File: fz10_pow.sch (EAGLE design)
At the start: 83 parts

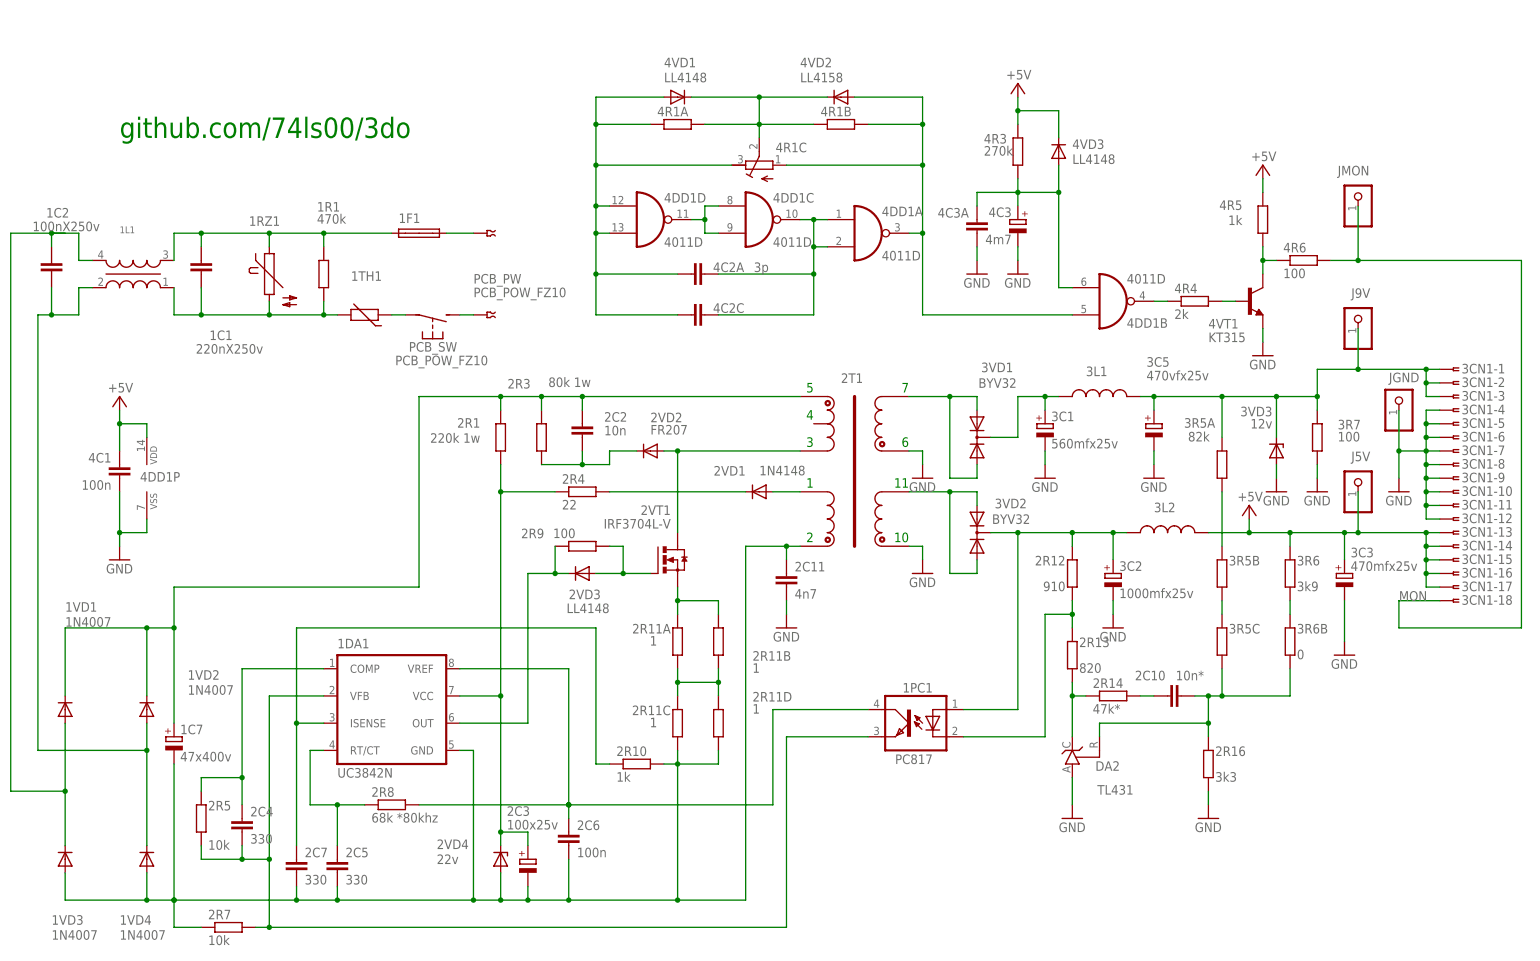
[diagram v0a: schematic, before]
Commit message: .
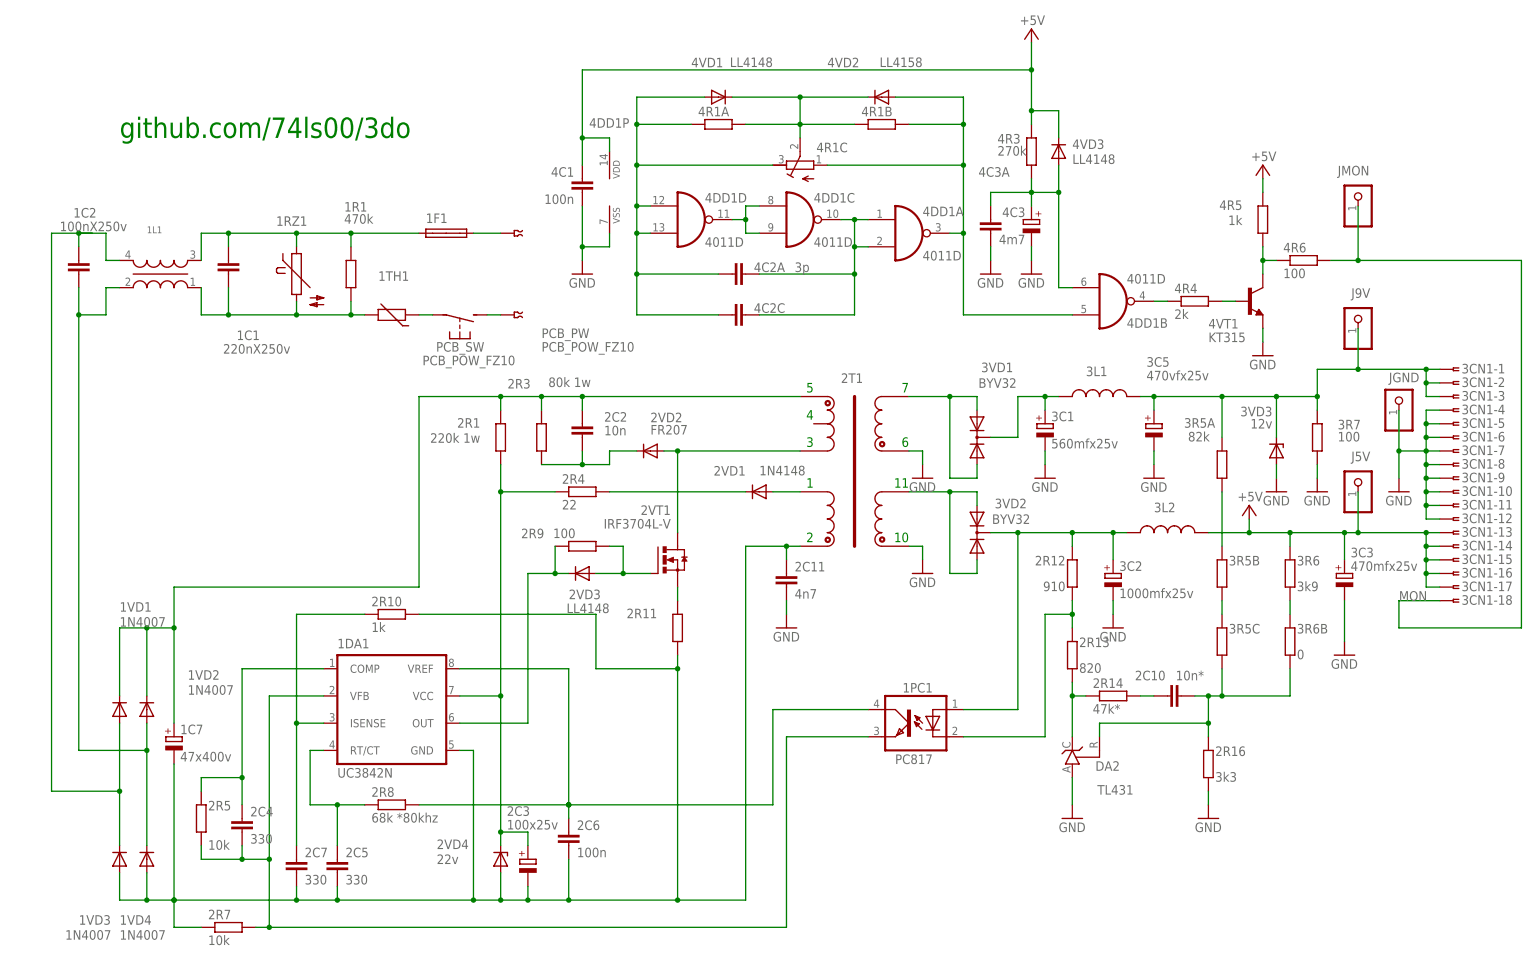
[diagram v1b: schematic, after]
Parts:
- removed 2R11A, 2R11B, 2R11C, 2R11D: 1, rcl:R-EU_R0805
- added 2R11: (no value), rcl:R-EU_0613/15
- 2VD1: device diode:1N4148DO35-7 -> diode:1N4148DO35-10
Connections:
- removed net N$21: 2R11A.2, 2R11B.2, 2VT1.S
- net -IN: now also 2R11.1; no longer 2R11C.1, 2R11D.1
- net N$37: now also 2R11.2, 2VT1.S; no longer 2R11A.1, 2R11B.1, 2R11C.2, 2R11D.2
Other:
- moved on the sheet: 1C1, 1C2, 1F1, 1L1, 1R1, 1RZ1, 1TH1, 1VD1, 1VD3, 2R10, 4C1, 4C2A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

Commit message: .
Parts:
- 2C11: device rcl:C-EU050-025X075 -> rcl:C-EU075-032X103
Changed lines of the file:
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@@
 <part name="2VD1" library="diode" deviceset="1N4148" device="DO35-10" value="1N4148"/>
 <part name="2R4" library="rcl" deviceset="R-EU_" device="0204/7" value="22"/>
-<part name="2C11" library="rcl" deviceset="C-EU" device="050-025X075" value="4n7"/>
+<part name="2C11" library="rcl" deviceset="C-EU" device="075-032X103" value="4n7"/>
 <part name="GND4" library="supply1" deviceset="GND" device=""/>
 <part name="1F1" library="fuse" deviceset="SHK20L" device=""/>
